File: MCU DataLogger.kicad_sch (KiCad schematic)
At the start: 25 parts, among them U1 24LC1025, U2 24LC1025, U3 DS1337S+, U4 ATMEGA328P-AU, Y1 32.768 KHz, Y2 16 MHz

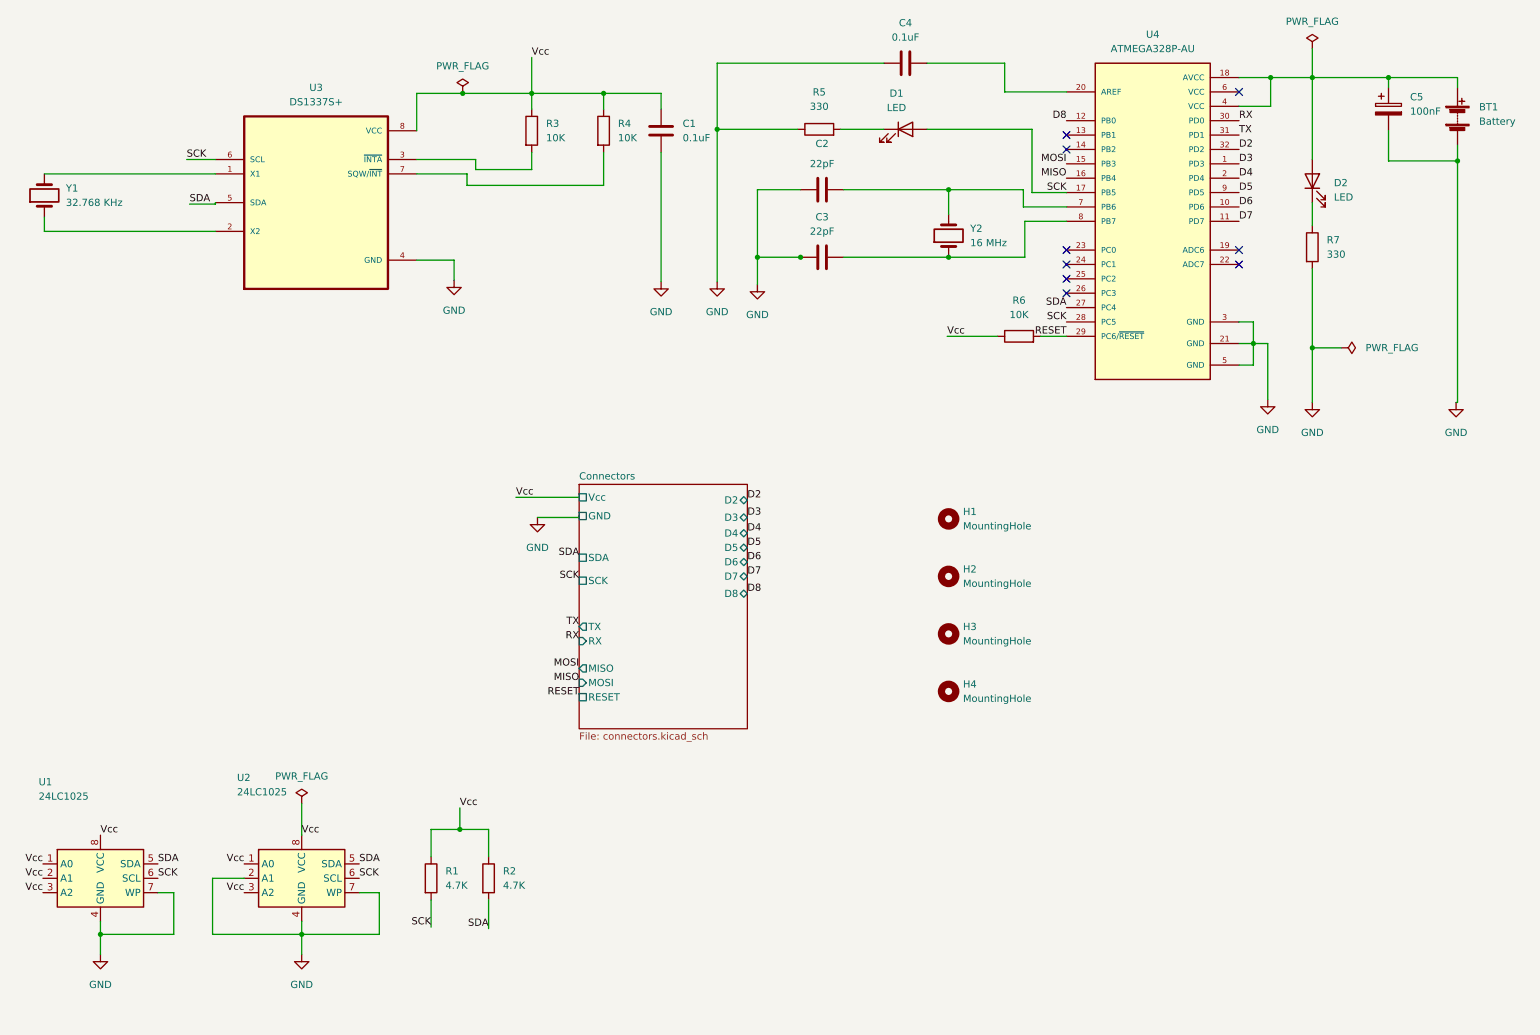
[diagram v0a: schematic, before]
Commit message: Completed comments.
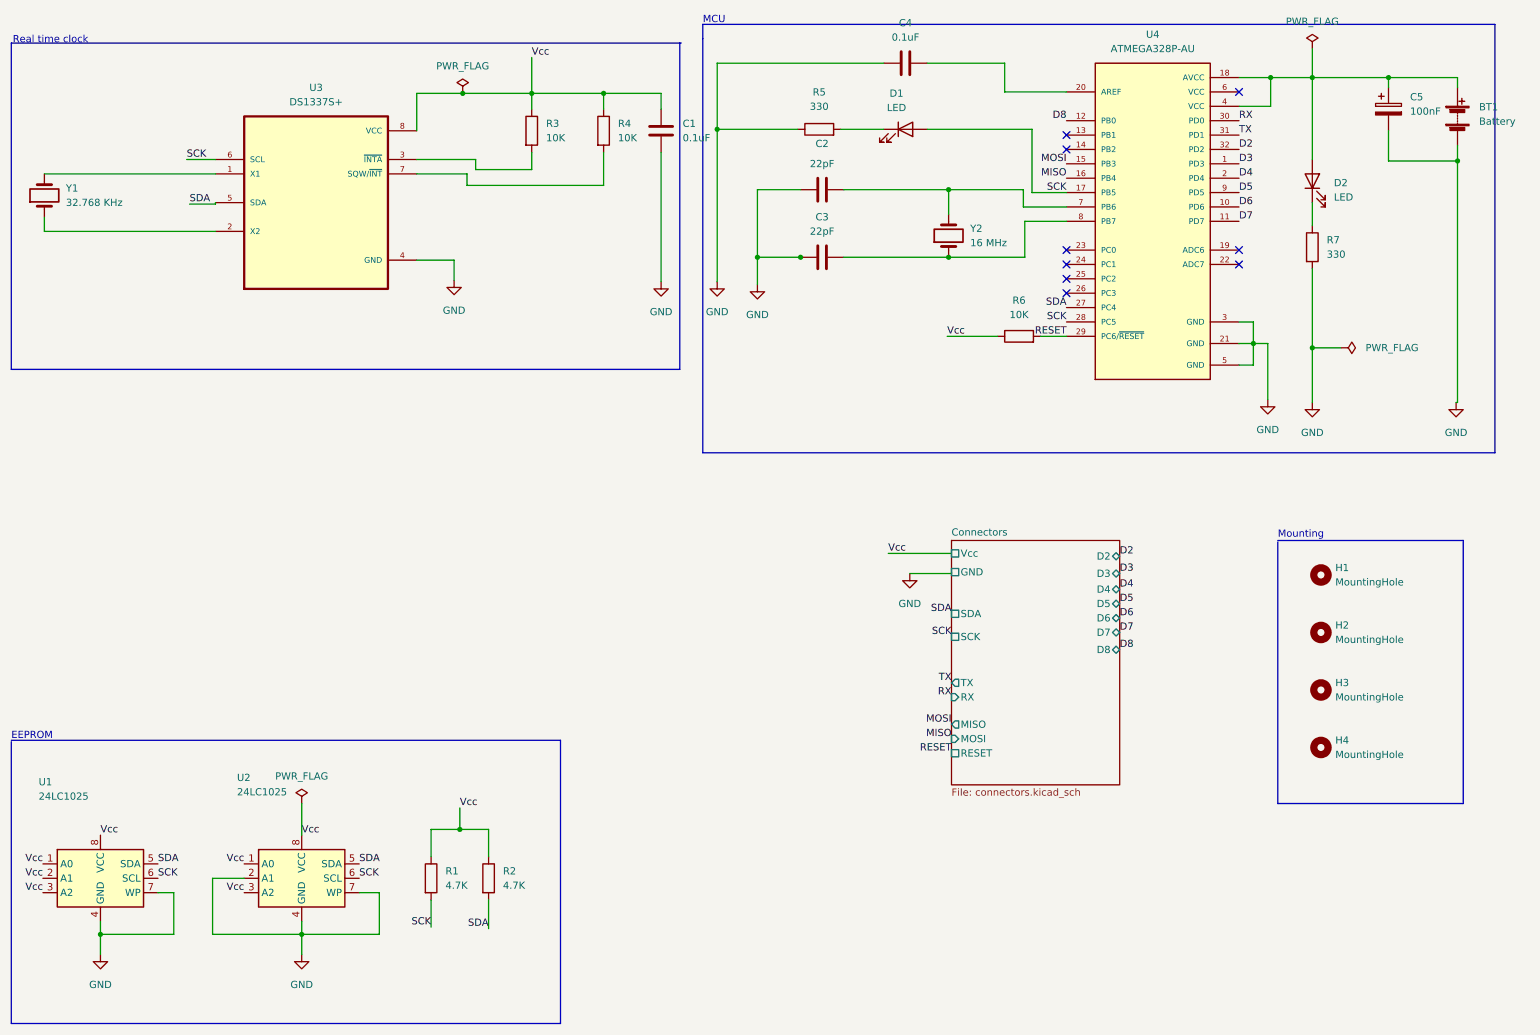
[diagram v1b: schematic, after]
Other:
- note added: "EEPROM"
- note added: "MCU"
- note added: "Mounting"
- note added: "Real time clock"
- moved on the sheet: H1, H2, H3, H4
